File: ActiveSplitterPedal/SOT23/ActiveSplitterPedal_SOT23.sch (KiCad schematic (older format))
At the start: 18 parts, among them J1 MonoJack2Switch, J2 MonoJack2Switch, J3 MonoJack2Switch, J4 MonoJack2Switch, J5 MonoJack2Switch, J6 Barrel_Jack, SW1 SW_DIP_x04

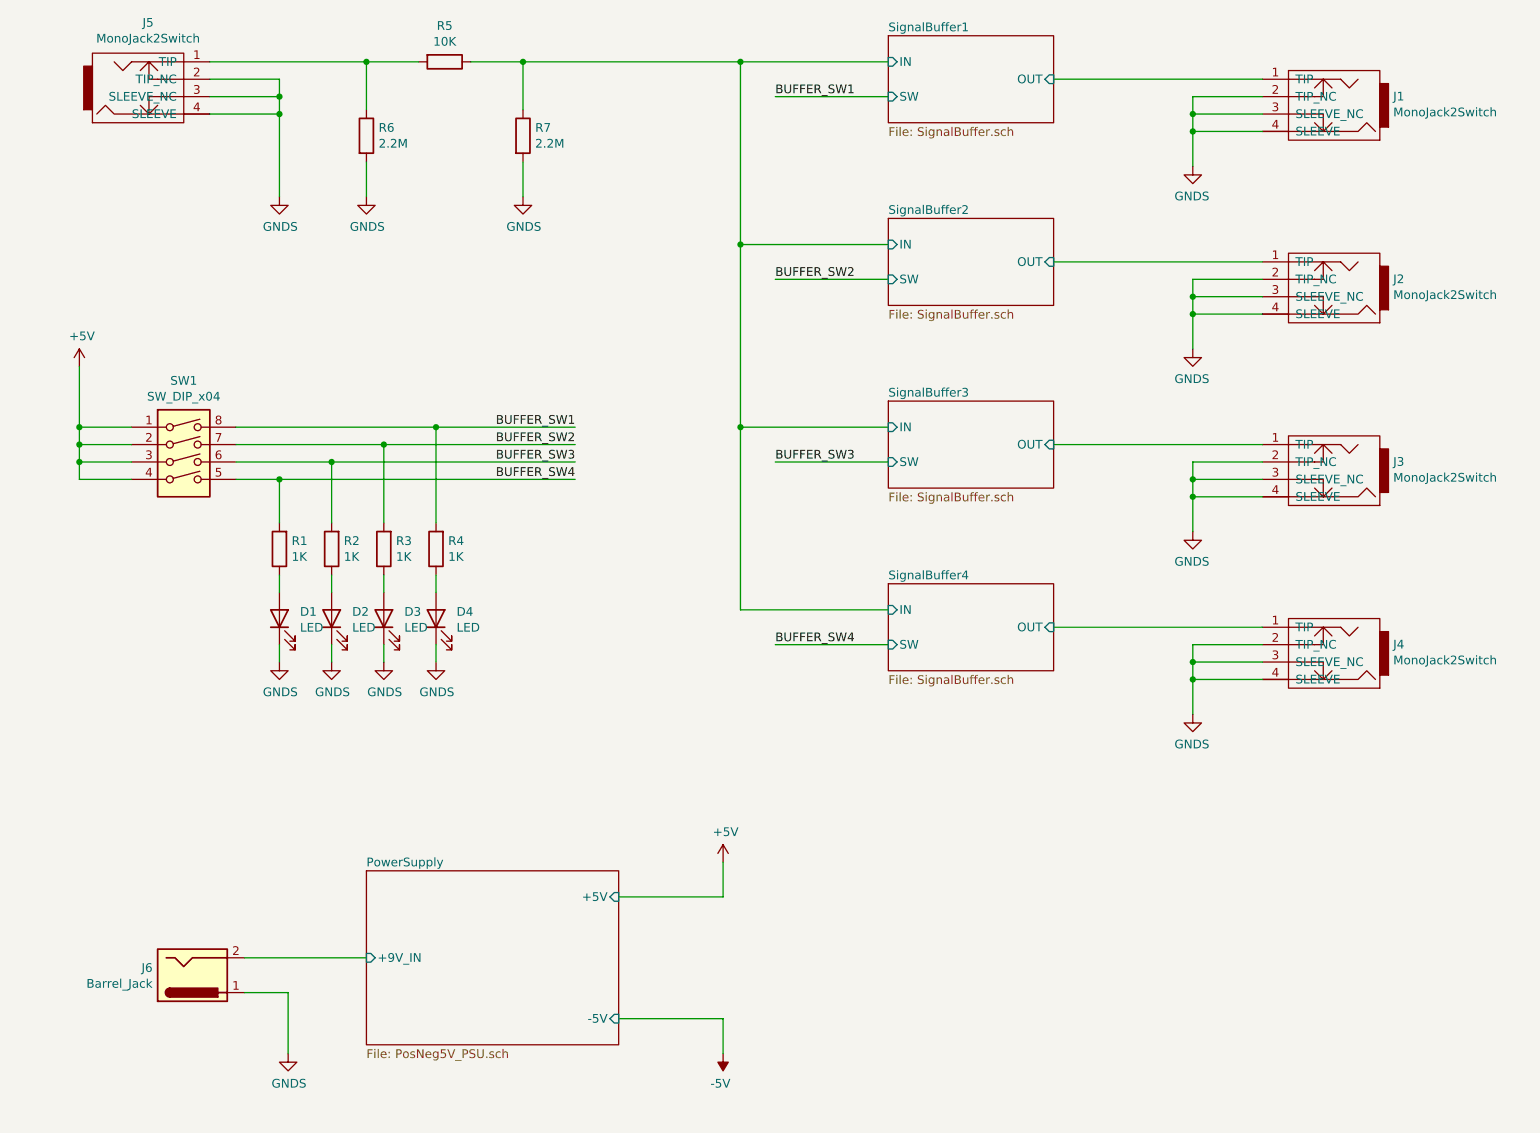
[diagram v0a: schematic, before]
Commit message: updated schematic
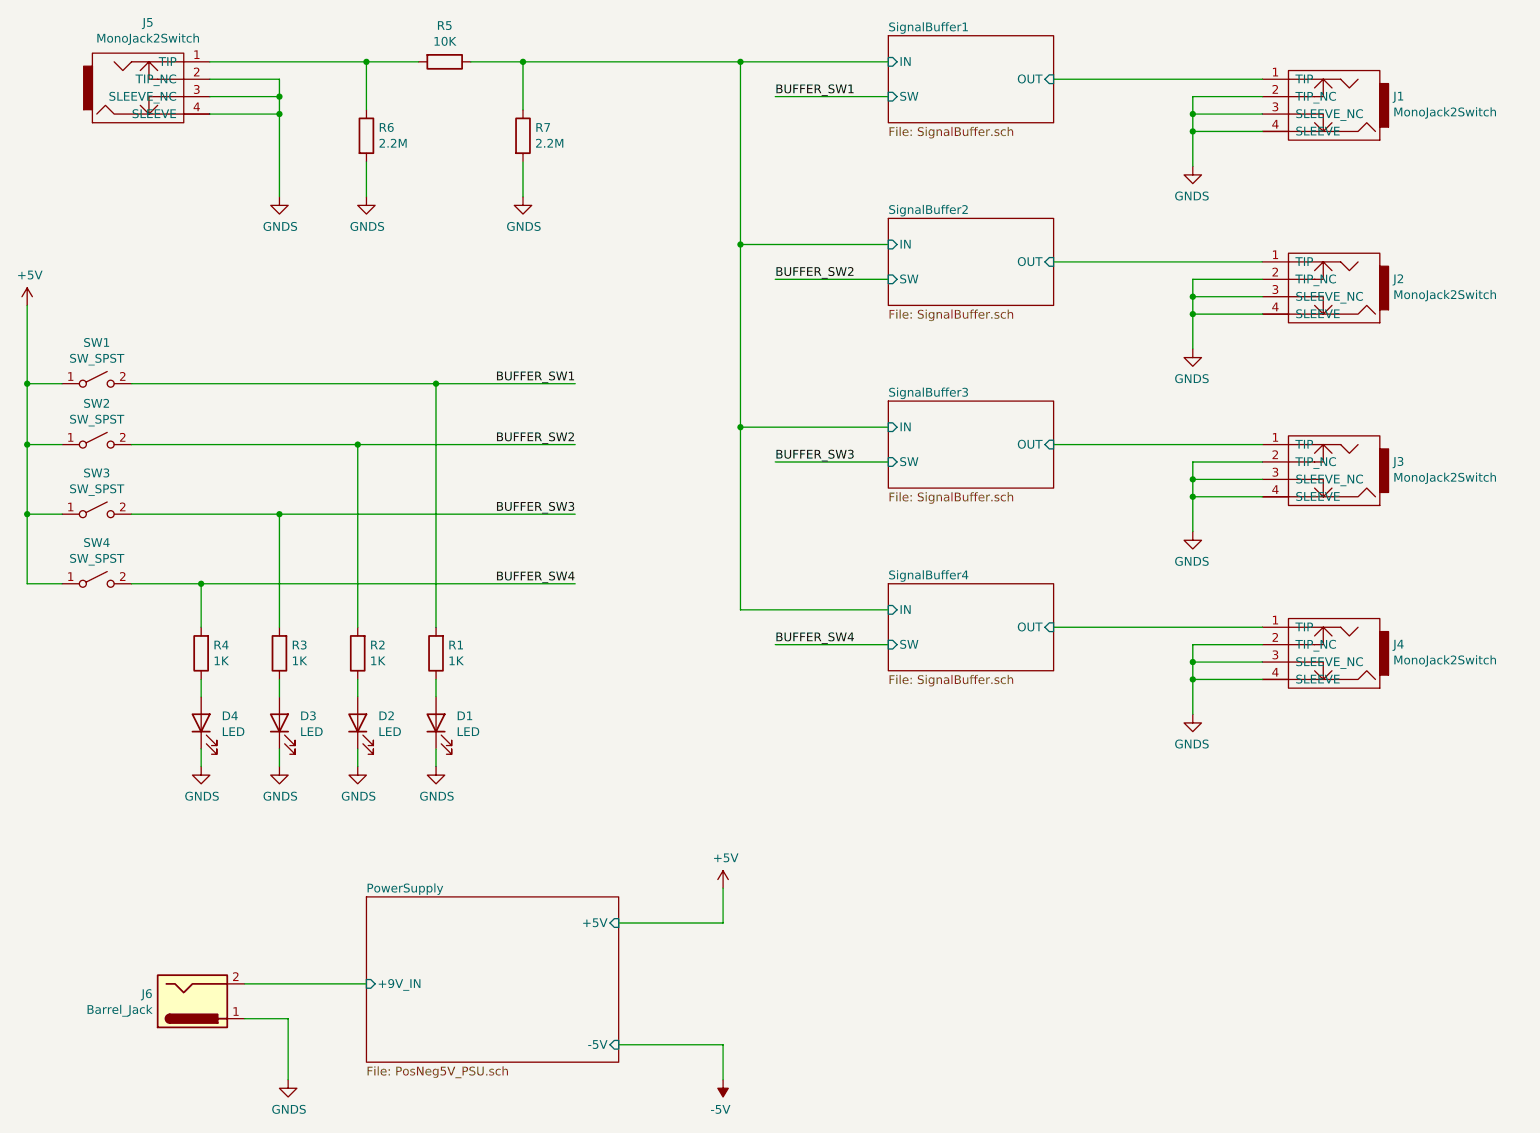
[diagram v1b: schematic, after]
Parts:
- removed SW1: SW_DIP_x04, Button_Switch_SMD:SW_DIP_SPSTx04_Slide_6.7x11.72mm_W6.73mm_P2.54mm_LowProfile_JPin, symbol Switch:SW_DIP_x04
- added SW1, SW2, SW3, SW4: SW_SPST, Connector_PinHeader_2.54mm:PinHeader_1x02_P2.54mm_Vertical, symbol Switch:SW_SPST
- D1, D2, D3, D4: footprint LED_SMD:LED_0805_2012Metric_Pad1.15x1.40mm_HandSolder -> LED_THT:LED_D5.0mm
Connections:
- net +5V: now also SW1.1 (A), SW2.1 (A), SW3.1 (A), SW4.1 (A)
- net BUFFER_SW1: now also R1.2, SW1.2 (B); no longer R4.2
- net BUFFER_SW2: now also R2.2, SW2.2 (B); no longer R3.2
- net BUFFER_SW3: now also R3.2, SW3.2 (B); no longer R2.2
- net BUFFER_SW4: now also R4.2, SW4.2 (B); no longer R1.2
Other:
- moved on the sheet: D1, D2, D3, D4, J6, R1, R2, R3, R4
